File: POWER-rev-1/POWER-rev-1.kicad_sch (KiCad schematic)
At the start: 93 parts, among them SW1 EG25-switch-CSS-1210MC, SW2 MIC-switch-CSS-1210MC, SW3 CAM-switch-CSS-1210MC, U1 BAT-CONNECTOR-FLTS22WR00, U2 MP3429GL-Z, U3 BQ25792RQMR, U4 22V-boost-AP3032KTR-G1, U5 TPS65023BRSBR

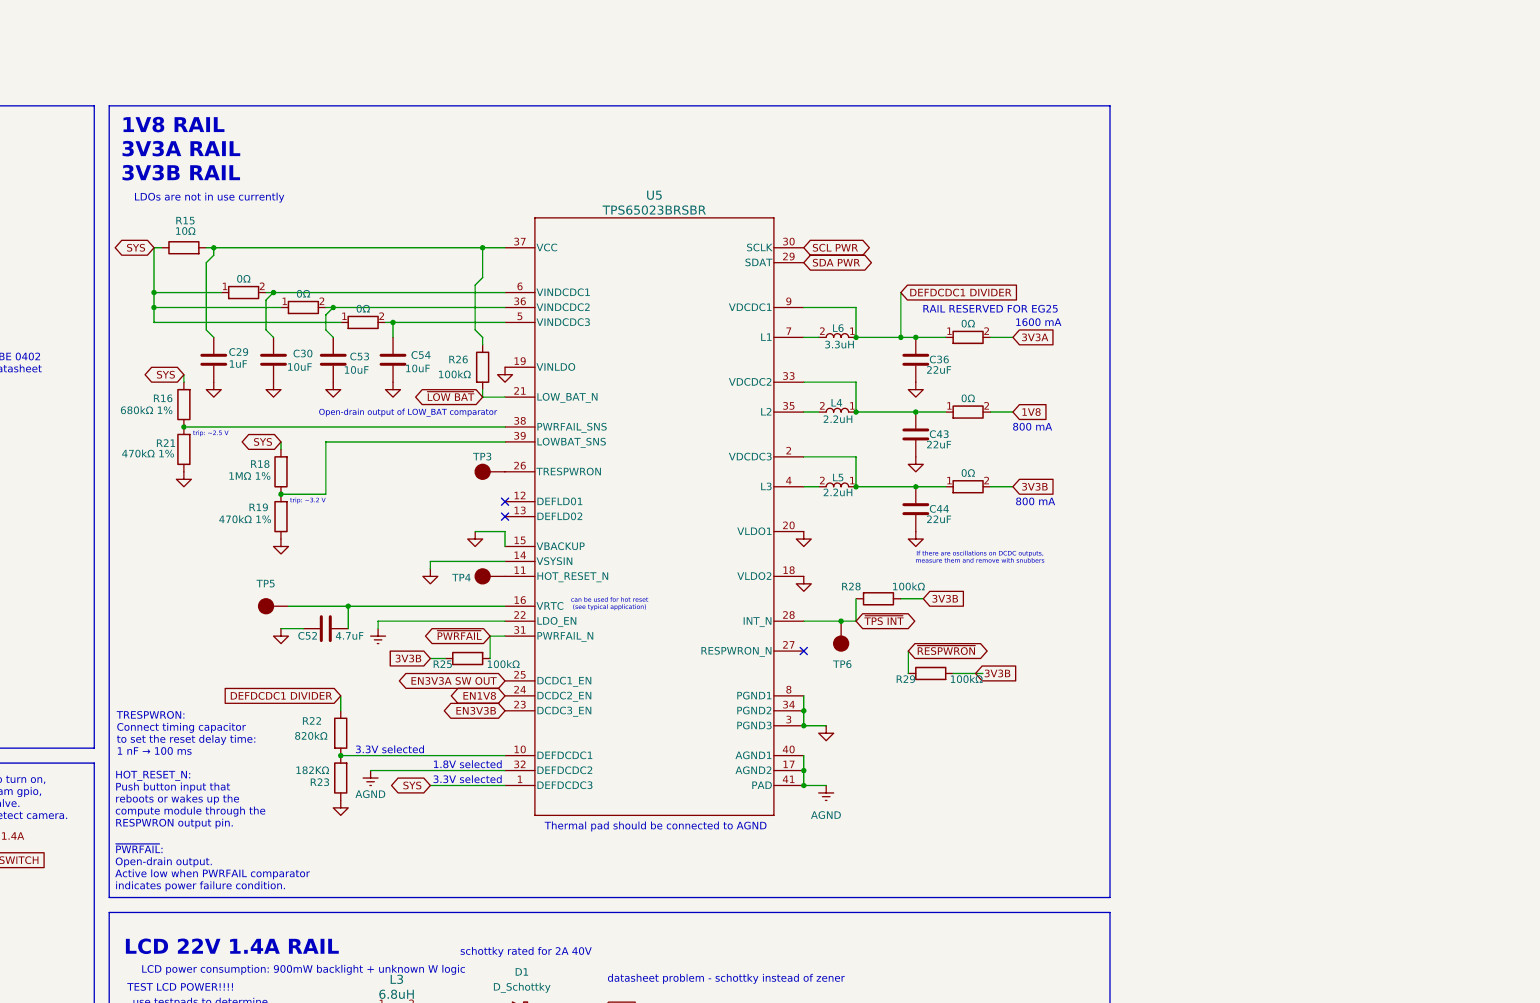
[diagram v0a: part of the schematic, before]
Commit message: replace 0ohm resistors with jumpers
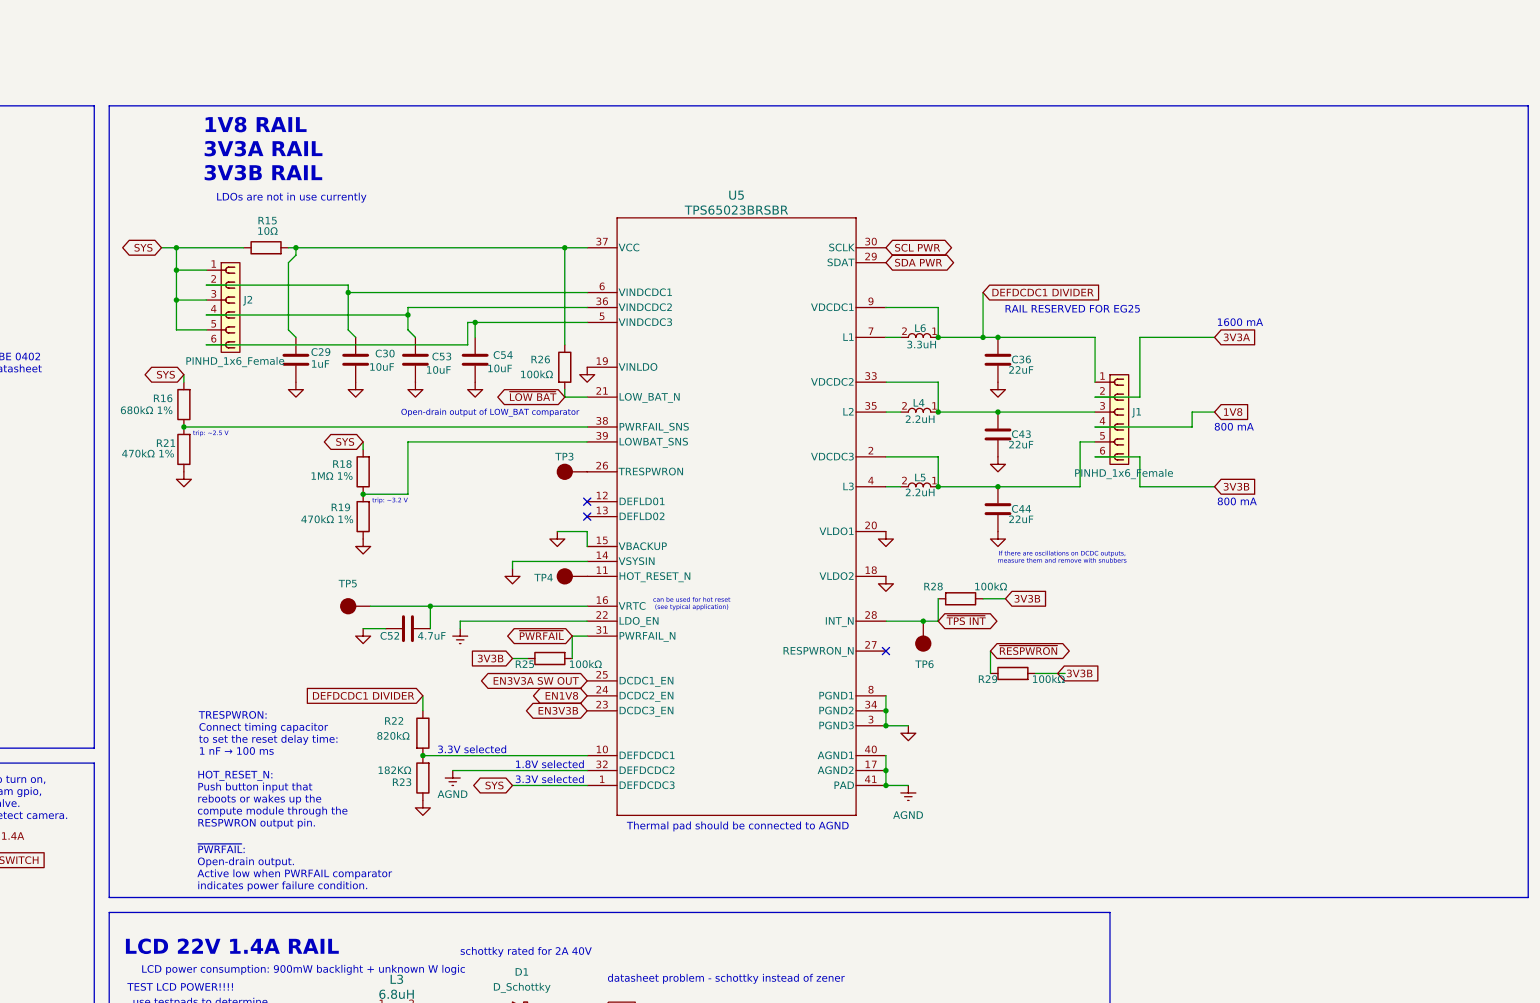
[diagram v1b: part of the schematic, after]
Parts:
- removed R17, R20, R24: 0Ω, SPIRIT-footprints:1K-05W-0805-RES_ERJP06J102V, symbol SPIRIT-components:1K-05W-0805-RES_ERJP06J102V
- removed R30, R31, R32: 0Ω, SPIRIT-footprints:0805-resistor, symbol SPIRIT-components:1K-05W-0805-RES_ERJP06J102V
- added J1, J2: PINHD_1x6_Female, SL_Connectors:PinHeader_1x06_P2.54mm_Vertical, symbol SL_Pin_Headers:PINHD_1x6_Female
- R15: footprint (none) -> SPIRIT-footprints:0805-resistor
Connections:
- net 1V8: now also J1.4
- net 3V3A: now also J1.2
- net 3V3B: now also J1.6
- net DEFDCDC1 DIVIDER: now also J1.1
- net SYS: now also J2.1, J2.3, J2.5
- net at C30.1, U5.6 (VINDCDC1): now also J2.2
- net at C44.1, L5.1, U5.2 (VDCDC3): now also J1.5
- net at C54.1, U5.5 (VINDCDC3): now also J2.6
- net at C53.1, U5.36 (VINDCDC2): now also J2.4
- net at C43.1, L4.1, U5.33 (VDCDC2): now also J1.3
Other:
- moved on the sheet: C29, C30, C36, C43, C44, C52, C53, C54, L4, L5, L6, R15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
